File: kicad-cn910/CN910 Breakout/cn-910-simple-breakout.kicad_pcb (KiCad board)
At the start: 2 copper layers, 24 x 20 mm, 21 parts, among them J1 CN910_FPC_CON, J2 J_PB_RF

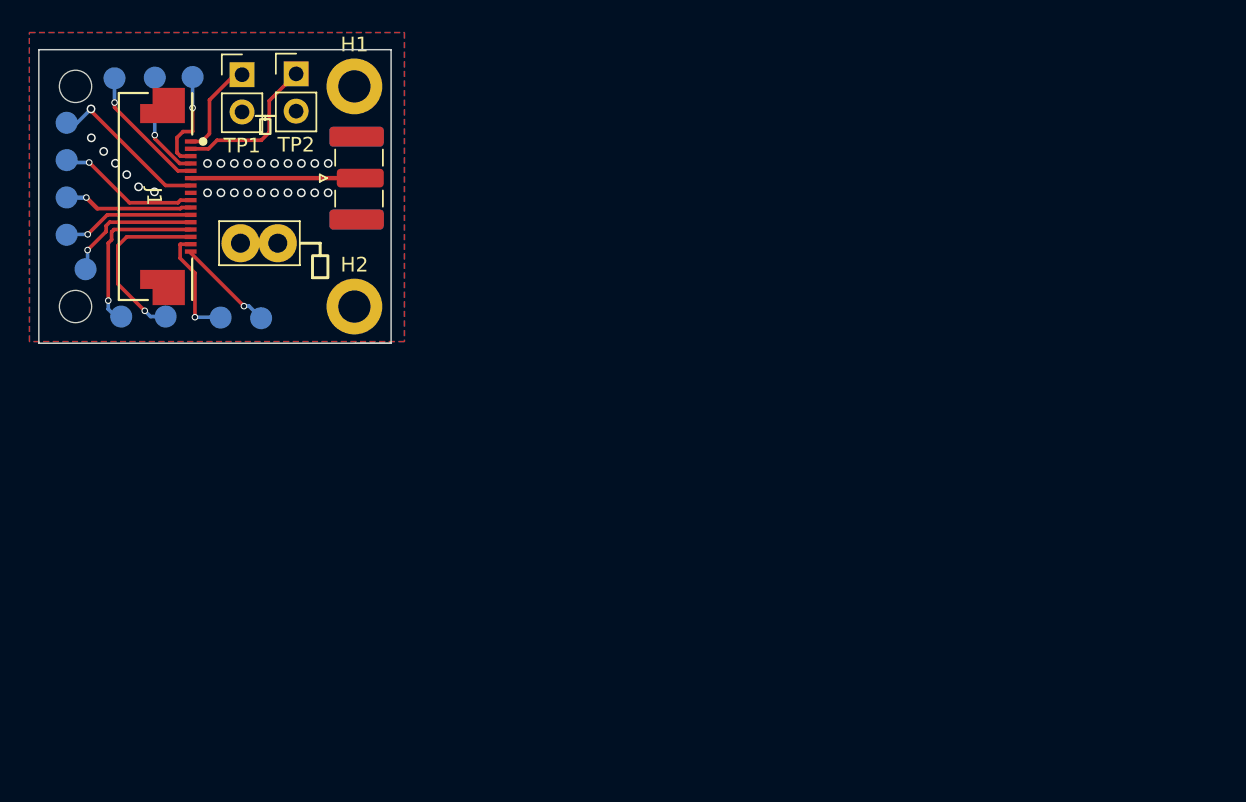
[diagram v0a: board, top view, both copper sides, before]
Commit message: Refactor code structure for improved readability and maintainability
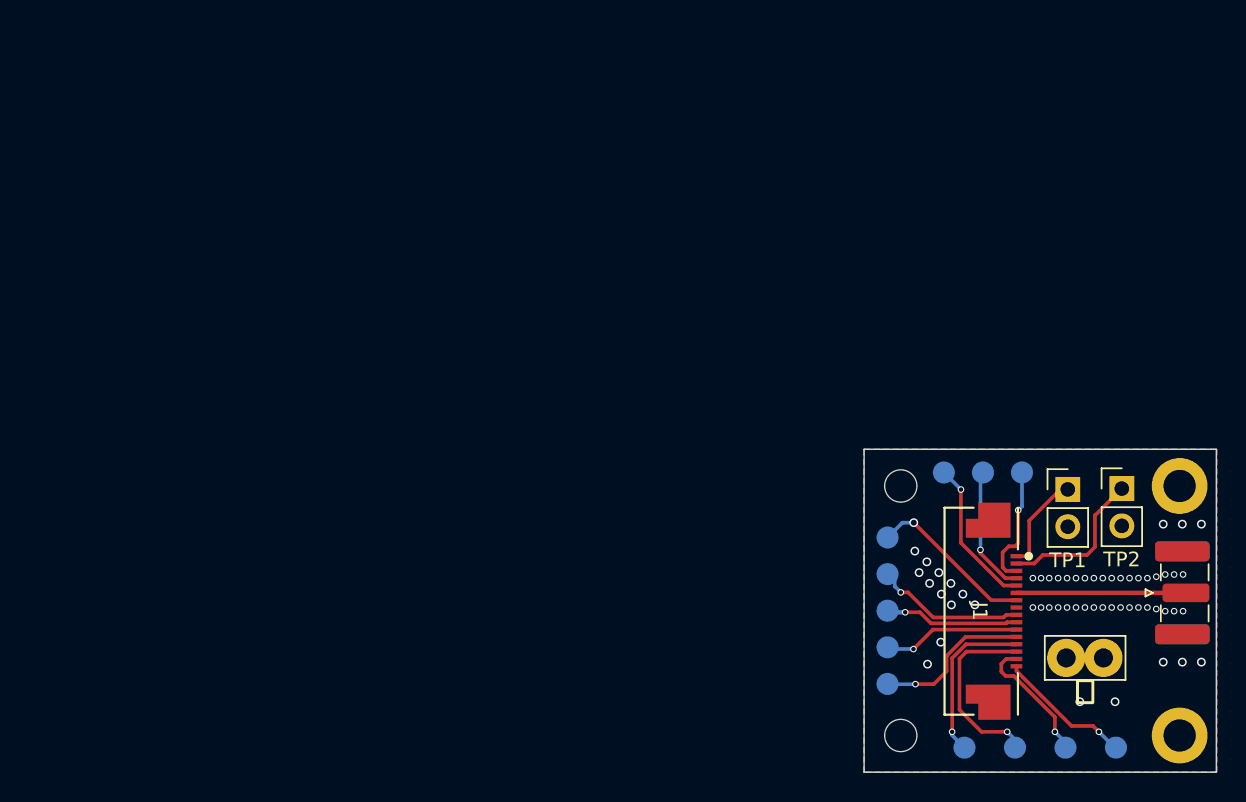
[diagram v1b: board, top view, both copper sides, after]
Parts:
- added SONY_SIMPLE**: Board, PCM_kikit:Board, F.Cu at (196.3, 112.4)
- moved TP16 65.2 mm to (213.5, 132.7), turned to -105 degrees
- moved TP14 64.9 mm to (206.6, 132.7)
- moved TP15 64.6 mm to (210.0, 132.7), turned to -135 degrees
- moved TP13 64.5 mm to (203.2, 132.7)
- moved H2 63.4 mm to (217.8, 131.9)
- moved H4 63.4 mm to (198.8, 131.9)
- moved TP1 63.0 mm to (210.2, 115.1)
- moved J2 63.0 mm to (218.3, 122.2)
- moved TP8 63.0 mm to (212.6, 126.6)
- moved J1 63.0 mm to (204.3, 123.4)
- moved TP2 63.0 mm to (213.9, 115.1)
- moved TP7 62.7 mm to (197.9, 118.4)
- moved TP9 62.6 mm to (197.9, 120.9)
- moved TP10 62.6 mm to (197.9, 123.4)
- moved TP3 62.6 mm to (207.1, 114.0)
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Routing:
- net Net-(J1-EVF_VG): track 6.73 -> 9.27 mm
- net Net-(J1-AFC_F0): track 7.30 -> 8.73 mm
- net Net-(J1-IR_VIDEO): track 7.02 -> 8.39 mm
- net Net-(J1-CAP_FG): track 9.41 -> 10.7 mm
- net Net-(J1-BPF_MONI): track 8.97 -> 10.3 mm
- net Net-(J1-VCO): track 7.86 -> 9.05 mm
- net Net-(J1-EVF_BL_4.75V): track 12.0 -> 13.0 mm
- net Net-(J1-EVF_BL): track 11.9 -> 11.2 mm
- net GND: vias 26 -> 56
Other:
- board size 24 x 20 mm -> 24 x 22 mm
